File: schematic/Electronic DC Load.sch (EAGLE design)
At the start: 93 parts, among them J1 POWER_JACKPTH_LOCK, J2 AVR_SPI_PROG_3X22X3_LOCK, Q1 IRFP250NH, Q2 600mA/40V, U1 ATMEGA328P_TQFP, U2 PCF8574_DW_16, U3 REF5050_D_8, U4 INA210AIDCKRG4, U5 MP1584EN, U6 AD8629ARZ, U7 AD7190BRUZ, U8 AD5541ARZ, U9 LM35_LP_3, Y1 16MHz

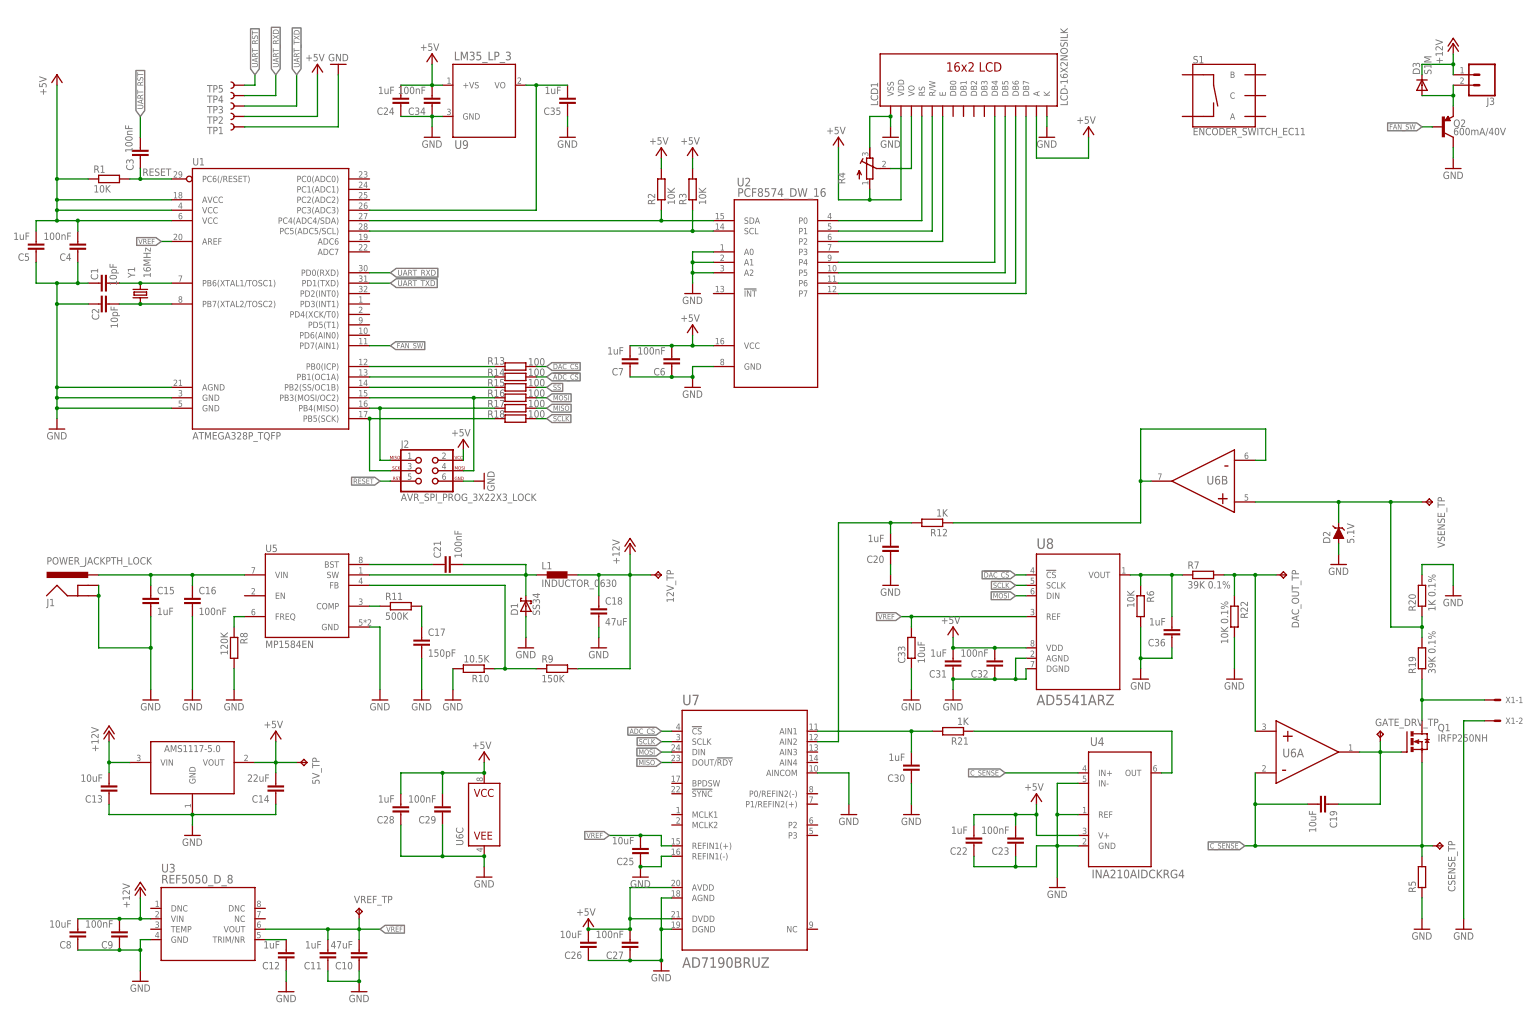
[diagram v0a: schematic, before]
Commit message: First layouts
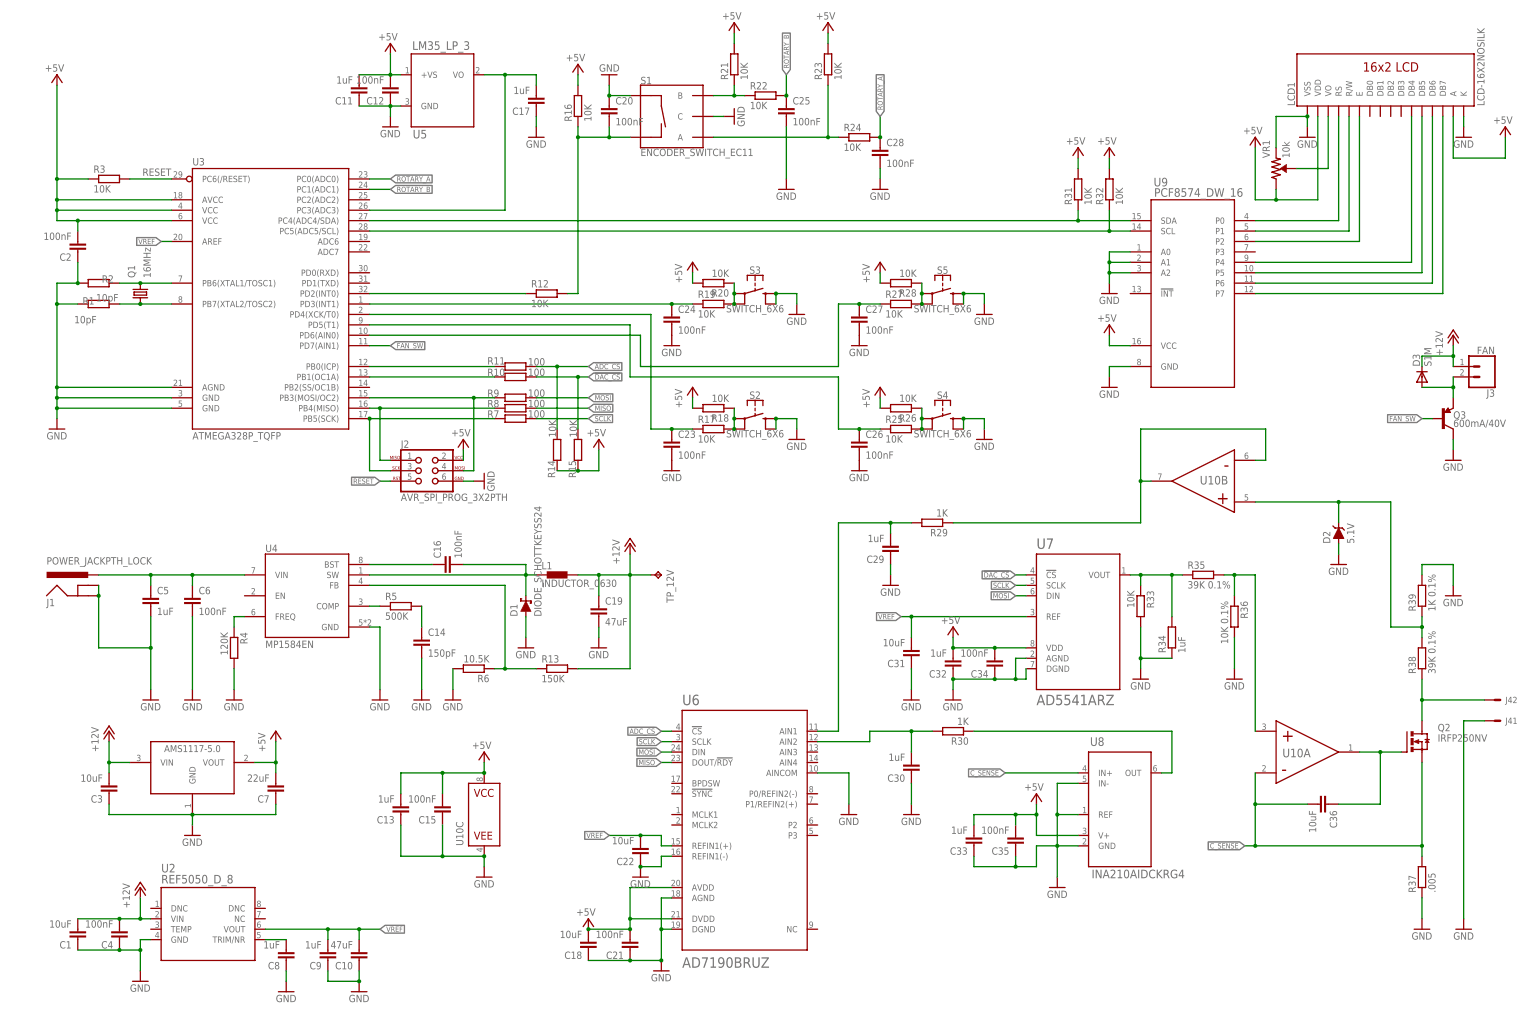
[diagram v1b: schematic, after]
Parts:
- removed 5V_TP, CSENSE_TP, DAC_OUT_TP, GATE_DRV_TP, VREF_TP, VSENSE_TP: TPB2,54, testpad:TPB2,54
- removed TP1: TEST-POINT2, SparkFun-Connectors:TEST-POINT2
- removed TP2, TP3, TP4, TP5: TEST-POINT3, SparkFun-Connectors:TEST-POINT3
- removed U$1: AMS1117-5.0, AMS1117-5.0:AMS1117-5.0
- removed X1: (no value), con-molex:KK-156-2
- removed Y1: 16MHz, crystal-geyer_V1_0:KX-7
- added J4: KF762-2, 0_discrete:KF762-2
- added Q3: 600mA/40V, SparkFun-DiscreteSemi:TRANS_PNP-MMBT4403
- added R23, R24, R25, R26, R27, R28, R31, R32, R33: 10K, resistor:R-EU_R0603
- added R29, R30: 1K, resistor:R-EU_R0805
- added R34: 1uF, resistor:R-EU_R0805
- added R35: 39K 0.1%, resistor:R-EU_R0805
- added R36: 10K 0.1%, resistor:R-EU_R0805
- added R37: .005, 0_sup:MRE_R005_4W_2728_1%
- added R38: 39K 0.1%, resistor:R-EU_M0805
- added R39: 1K 0.1%, resistor:R-EU_M0805
- added S2, S3, S4, S5: SWITCH_6X6, 0_discrete:SWITCH_6X6
- added U10: AD8629ARZ, 0_analog-devices:AD8629ARZ
- added VR1: 10k, SparkFun-Resistors:TRIMPOT-SMD-3MM-OPEN-1/10W-25%
- C1: value 10pF -> 10uF; device resistor:C-EUC0603 -> resistor:C-EUC1206
- C10: device resistor:C-EUC0603 -> resistor:C-EUC1206
- C11, C34, C4, C5, C6: device resistor:C-EUC0603 -> resistor:C-EUC0805
- C12, C35: value 1uF -> 100nF; device resistor:C-EUC0603 -> resistor:C-EUC0805
- C13, C8: value 10uF -> 1uF; device resistor:C-EUC0603 -> resistor:C-EUC0805
- C14: value 22uF -> 150pF; device resistor:C-EUC0603 -> resistor:C-EUC0402
- C15, C24: value 1uF -> 100nF
- C17: value 150pF -> 1uF; device resistor:C-EUC1206 -> resistor:C-EUC0805
- C18: value 47uF -> 10uF
- C19: value 10uF -> 47uF; device resistor:C-EUC0603 -> resistor:C-EUC1206
- C2: value 10pF -> 100nF
- C20, C28: value 1uF -> 100nF; device resistor:C-EUC0805 -> resistor:C-EUC0603
- C21: device resistor:C-EUC1206 -> resistor:C-EUC0805
- C22: value 1uF -> 10uF; device resistor:C-EUC0805 -> resistor:C-EUC1206
- C23: device resistor:C-EUC0805 -> resistor:C-EUC0603
- C25, C26: value 10uF -> 100nF
- C29: value 100nF -> 1uF
- C3: value 100nF -> 10uF; device resistor:C-EUC0603 -> resistor:C-EUC1206
- C31, C36: value 1uF -> 10uF; device resistor:C-EUC0603 -> resistor:C-EUC1206
- C32, C9: value 100nF -> 1uF; device resistor:C-EUC0603 -> resistor:C-EUC0805
- C33: value 10uF -> 1uF; device resistor:R-EU_M1206 -> resistor:C-EUC0805
- C7: value 1uF -> 22uF; device resistor:C-EUC0603 -> resistor:C-EUC1206
- D1: value SS34 -> DIODE_SCHOTTKEYSS24; device diode:SCHOTTKY-DIODESMC -> 0_discrete:DIODE_SCHOTTKEYSS24
- J2: value AVR_SPI_PROG_3X22X3_LOCK -> AVR_SPI_PROG_3X2PTH; device SparkFun-Connectors:AVR_SPI_PROG_3X22X3_LOCK -> SparkFun-Connectors:AVR_SPI_PROG_3X2PTH
- J3: value (none) -> FAN
- Q1: value IRFP250NH -> 16MHz; device 0_discrete:IRFP250NH -> crystal-geyer_V1_0:KX-7
- Q2: value 600mA/40V -> IRFP250NV; device SparkFun-DiscreteSemi:TRANS_PNP-MMBT4403 -> 0_discrete:IRFP250NV
- R1, R2: value 10K -> 10pF; device resistor:R-EU_R0603 -> resistor:R-EU_R0805
- R10: value 10.5K -> 100; device resistor:R-EU_R0603 -> resistor:R-EU_M0805
- R11: value 500K -> 100; device resistor:R-EU_R0603 -> resistor:R-EU_M0805
- R12, R21: value 1K -> 10K; device resistor:R-EU_R0805 -> resistor:R-EU_R0603
- R13: value 100 -> 150K; device resistor:R-EU_M0805 -> resistor:R-EU_R0603
- R14, R15: value 100 -> 10K
- R16, R17, R18: value 100 -> 10K; device resistor:R-EU_M0805 -> resistor:R-EU_R0603
- R19: value 39K 0.1% -> 10K; device resistor:R-EU_M0805 -> resistor:R-EU_R0603
- R20: value 1K 0.1% -> 10K; device resistor:R-EU_M0805 -> resistor:R-EU_R0603
- R22: value 10K 0.1% -> 10K; device resistor:R-EU_R0805 -> resistor:R-EU_R0603
- R4: value (none) -> 120K; device resistor:R-TRIMM3296P -> resistor:R-EU_R0603
- R5: value (none) -> 500K; device 0_sup:MRE_R005_4W_2728_1% -> resistor:R-EU_R0603
- R6: value 10K -> 10.5K; device resistor:R-EU_R0805 -> resistor:R-EU_R0603
- R7: value 39K 0.1% -> 100; device resistor:R-EU_R0805 -> resistor:R-EU_M0805
- R8: value 120K -> 100; device resistor:R-EU_R0603 -> resistor:R-EU_M0805
- R9: value 150K -> 100; device resistor:R-EU_R0603 -> resistor:R-EU_M0805
- U1: value ATMEGA328P_TQFP -> AMS1117-5.0; device SparkFun-IC-Microcontroller:ATMEGA328P_TQFP -> AMS1117-5.0:AMS1117-5.0
- U2: value PCF8574_DW_16 -> REF5050_D_8; device 0_texas-instrument:PCF8574_DW_16 -> 0_texas-instrument:REF5050_D_8
- U3: value REF5050_D_8 -> ATMEGA328P_TQFP; device 0_texas-instrument:REF5050_D_8 -> SparkFun-IC-Microcontroller:ATMEGA328P_TQFP
- U4: value INA210AIDCKRG4 -> MP1584EN; device 0_texas-instrument:INA210AIDCKRG4 -> MP1584EN:MP1584EN
- U5: value MP1584EN -> LM35_LP_3; device MP1584EN:MP1584EN -> 0_texas-instrument:LM35_LP_3
- U6: value AD8629ARZ -> AD7190BRUZ; device 0_analog-devices:AD8629ARZ -> 0_analog-devices:AD7190BRUZ
- U7: value AD7190BRUZ -> AD5541ARZ; device 0_analog-devices:AD7190BRUZ -> 0_analog-devices:AD5541ARZ
- U8: value AD5541ARZ -> INA210AIDCKRG4; device 0_analog-devices:AD5541ARZ -> 0_texas-instrument:INA210AIDCKRG4
- U9: value LM35_LP_3 -> PCF8574_DW_16; device 0_texas-instrument:LM35_LP_3 -> 0_texas-instrument:PCF8574_DW_16
- renumbered 12V_TP to TP_12V
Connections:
- removed net !SS: R15.2
- removed net N$33: R15.1, U1.PB2(SS/OC1B)
- removed net UART_RST: C3.2, TP5.1
- removed net UART_RXD: TP4.1, U1.PD0(RXD)
- removed net UART_TXD: TP3.1, U1.PD1(TXD)
- removed net VCC: C4.2, C5.2, R1.1, TP2.1, U1.AVCC, U1.VCC@4, U1.VCC@6
- new net N$29: R21.1, R22.1, S1.B
- new net N$38: R23.1, R24.1, S1.A
- new net N$40: R17.2, R18.1, S2.1, S2.2
- new net N$41: R19.2, R20.1, S3.1, S3.2
- new net N$42: C20.2, R12.2, R16.1, S1.SW-
- new net N$43: C23.1, R17.1, U3.PD4(XCK/T0)
- new net N$44: R12.1, U3.PD2(INT0)
- new net N$46: C24.1, R19.1, U3.PD3(INT1)
- new net N$48: R27.2, R28.1, S5.1, S5.2
- new net N$51: R25.2, R26.1, S4.1, S4.2
- new net N$52: C26.1, R25.1, U3.PD5(T1)
- new net N$55: C27.1, R27.1, U3.PD6(AIN0)
- new net ROTARY_A: C28.1, R24.2, U3.PC0(ADC0)
- new net ROTARY_B: C25.1, R22.2, U3.PC1(ADC1)
- net !ADC_CS: now also R11.2, U6.!CS; no longer U7.!CS
- net !DAC_CS: now also R10.2, R15.2, U7.!CS; no longer R13.2, U8.!CS
- net +12V: now also C1.2, C19.1, C3.2, C4.2, R13.2, U1.VIN, U2.VIN; no longer C13.2, C18.1, C8.2, C9.2, R9.2, U$1.VIN, U3.VIN
- net +5V: now also C11.2, C12.2, C13.2, C15.2, C18.2, C2.2, C21.2, C33.2, C35.2, R14.1, R15.1, R16.2, R18.2, R20.2, R21.2, R23.2, R26.2, R28.2, R3.1, R31.2, R32.2, U1.VOUT, U10C.VCC, U3.AVCC, U3.VCC@4, U3.VCC@6, U5.+VS, U6.AVDD, U6.DVDD, U7.VDD, U8.V+, U9.VCC, VR1.CW; no longer 5V_TP.TP, C14.2, C22.2, C23.2, C24.2, C26.2, C27.2, C28.2, C29.2, C31.2, C6.2, R2.2, R3.2, R4.A, U$1.VOUT, U2.VCC, U4.V+, U6C.VCC, U7.AVDD, U7.DVDD, U8.VDD, U9.+VS
- net C_SENSE: now also C36.2, Q2.S, R37.2, U10A.IN-, U8.IN+; no longer C19.2, CSENSE_TP.TP, Q1.S, R5.2, U4.IN+, U6A.IN-
- net FAN_SW: now also Q3.B, U3.PD7(AIN1); no longer Q2.B, U1.PD7(AIN1)
- net GND: now also C14.2, C15.1, C17.1, C18.1, C19.2, C21.1, C23.2, C24.2, C25.2, C26.2, C27.2, C28.2, C3.1, C5.2, C6.2, J41.S, Q3.C, R1.1, R2.1, R33.2, R34.1, R36.2, R37.1, R39.2, R4.2, S1.C, S1.SW+, S2.3, S2.4, S3.3, S3.4, S4.3, S4.4, S5.3, S5.4, U1.GND, U10C.VEE, U3.AGND, U3.GND@3, U3.GND@5, U6.AGND, U6.AINCOM, U6.DGND, U6.REFIN1(-), U8.GND, U8.IN-, U8.REF, U9.A0, U9.A1, U9.A2, VR1.CCW; no longer C14.1, C15.2, C16.2, C17.2, C18.2, C23.1, C24.1, C25.1, C26.1, C27.1, C28.1, C36.1, C5.1, C6.1, Q2.C, R10.2, R20.2, R22.2, R4.E, R5.1, R8.2, TP1.1, U$1.GND, U1.AGND, U1.GND@3, U1.GND@5, U2.A0, U2.A1, U2.A2, U3.GND, U4.IN-, U4.REF, U6C.VEE, U7.AINCOM, U7.REFIN1(-), U8.AGND, U8.DGND, X1-2.S
- net MISO: now also R8.2, U6.DOUT/!RDY; no longer R17.2, U7.DOUT/!RDY
- net MOSI: now also R9.2, U6.DIN; no longer R16.2, U8.DIN
- net N$1: now also R31.1, U3.PC4(ADC4/SDA), U9.SDA; no longer R2.1, U1.PC4(ADC4/SDA), U2.SDA
- net N$10: now also C8.2, U2.TRIM/NR; no longer C12.2, U3.TRIM/NR
- net N$11: now also Q1.2, R2.2, U3.PB6(XTAL1/TOSC1); no longer C1.2, U1.PB6(XTAL1/TOSC1), Y1.2
- net N$12: now also Q1.1, R1.2, U3.PB7(XTAL2/TOSC2); no longer C2.2, U1.PB7(XTAL2/TOSC2), Y1.1
- net N$13: now also VR1.WIPER; no longer R4.S
- net N$14: now also J42.S, Q2.D, R38.1; no longer Q1.D, R19.1, X1-1.S
- net N$15: now also C17.2, U3.PC3(ADC3), U5.VO; no longer C35.2, U1.PC3(ADC3), U9.VO
- net N$16: now also C29.2, R29.2, U6.AIN1; no longer C20.2, R12.2, U7.AIN2
- net N$17: now also R4.1, U4.FREQ; no longer R8.1, U5.FREQ
- net N$18: now also R30.1, U8.OUT; no longer R21.1, U4.OUT
- net N$19: now also C16.1, U4.BST; no longer C21.1, U5.BST
- net N$2: now also R32.1, U3.PC5(ADC5/SCL), U9.SCL; no longer R3.1, U1.PC5(ADC5/SCL), U2.SCL
- net N$20: now also C5.1, C6.1, U4.VIN; no longer C15.1, C16.1, U5.VIN
- net N$21: now also C16.2, U4.SW; no longer C21.2, U5.SW
- net N$22: now also R13.1, R6.1, U4.FB; no longer R10.1, R9.1, U5.FB
- net N$23: now also R5.1, U4.COMP; no longer R11.1, U5.COMP
- net N$24: now also R30.2, U6.AIN2; no longer R21.2, U7.AIN1
- net N$25: now also C14.1, R5.2; no longer C17.1, R11.2
- net N$26: now also R33.1, R34.2, R35.1, U7.VOUT; no longer C36.2, R6.1, R7.1, U8.VOUT
- net N$27: now also R29.1, U10B.IN-, U10B.OUT; no longer R12.1, U6B.IN-, U6B.OUT
- net N$28: now also Q3.E; no longer Q2.E
- net N$3: now also U9.P4; no longer U2.P4
- net N$30: now also R7.1, U3.PB5(SCK); no longer R18.1, U1.PB5(SCK)
- net N$31: now also R8.1, U3.PB4(MISO); no longer R17.1, U1.PB4(MISO)
- net N$32: now also R9.1, U3.PB3(MOSI/OC2); no longer R16.1, U1.PB3(MOSI/OC2)
- net N$34: now also R10.1, U3.PB1(OC1A); no longer R14.1, U1.PB1(OC1A)
- net N$35: now also R11.1, U3.PB0(ICP); no longer R13.1, U1.PB0(ICP)
- net N$36: now also C36.1, Q2.G, U10A.OUT; no longer C19.1, GATE_DRV_TP.TP, Q1.G, U6A.OUT
- net N$37: now also R38.2, R39.1, U10B.IN+; no longer R19.2, R20.1, U6B.IN+, VSENSE_TP.TP
- net N$39: now also R35.2, R36.1, U10A.IN+; no longer DAC_OUT_TP.TP, R22.1, R7.2, U6A.IN+
- net N$4: now also U9.P5; no longer U2.P5
- net N$5: now also U9.P6; no longer U2.P6
- net N$6: now also U9.P7; no longer U2.P7
- net N$7: now also U9.P0; no longer U2.P0
- net N$8: now also U9.P1; no longer U2.P1
- net N$9: now also U9.P2; no longer U2.P2
- net RESET: now also R3.2, U3.PC6(/RESET); no longer C3.1, R1.2, U1.PC6(/RESET)
- net SCLK: now also R7.2, U6.SCLK; no longer R18.2, U8.SCLK
- net VREF: now also C22.2, C31.2, C9.2, U2.VOUT, U3.AREF, U6.REFIN1(+), U7.REF; no longer C11.2, C25.2, C33.2, U1.AREF, U3.VOUT, U7.REFIN1(+), U8.REF, VREF_TP.TP
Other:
- moved on the sheet: C1, C11, C12, C13, C14, C15, C16, C17, C18, C19, C2, C20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
